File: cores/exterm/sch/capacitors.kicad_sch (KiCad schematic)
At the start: 27 parts

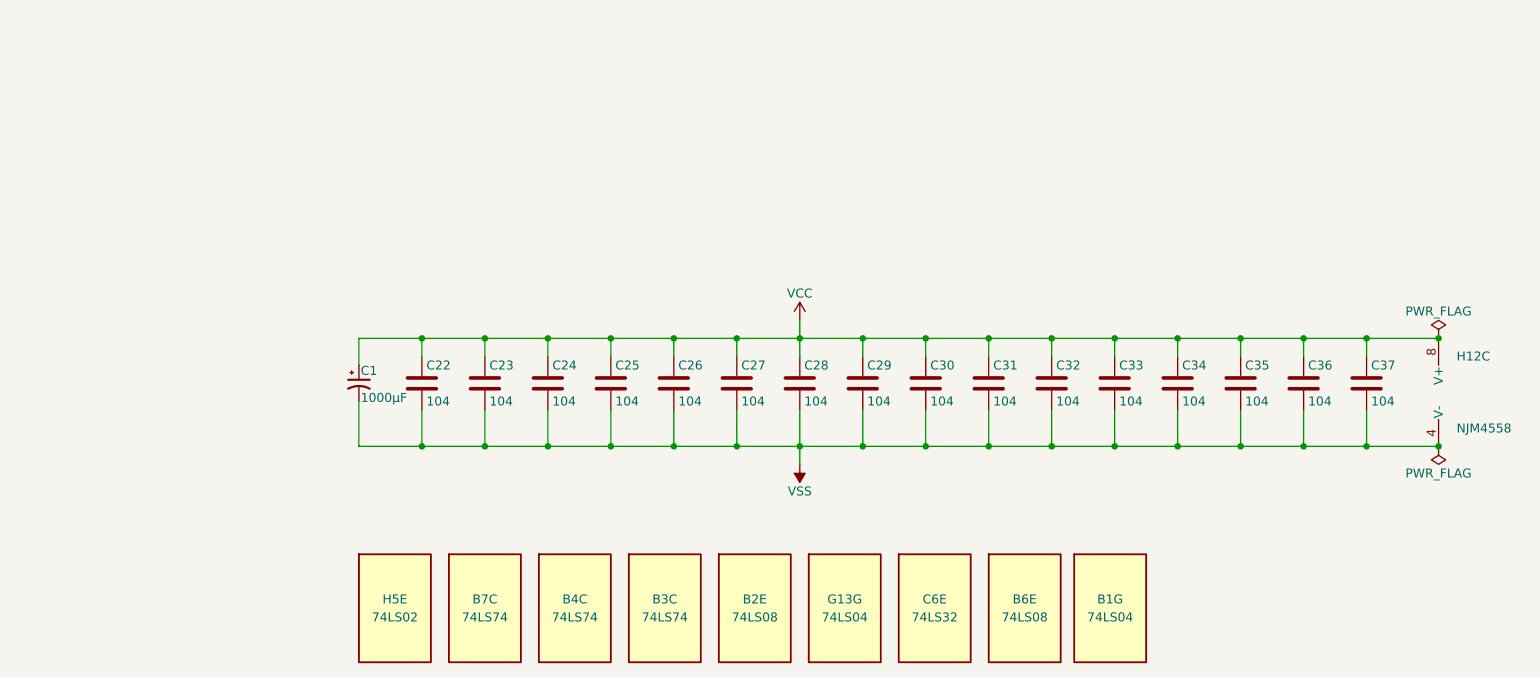
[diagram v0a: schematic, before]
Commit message: issues_exterm
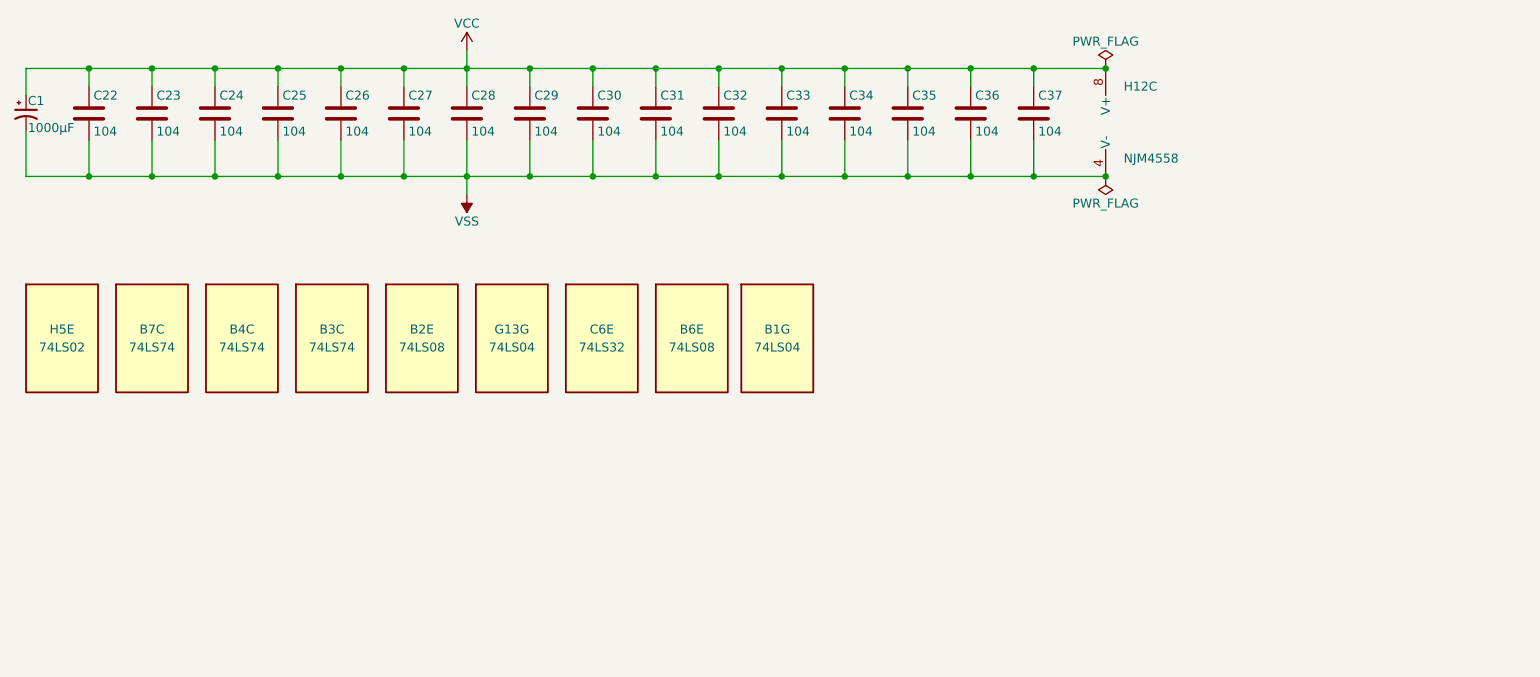
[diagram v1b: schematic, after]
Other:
- moved on the sheet: B1G, B2E, B3C, B4C, B6E, B7C, C1, C22, C23, C24, C25, C26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
